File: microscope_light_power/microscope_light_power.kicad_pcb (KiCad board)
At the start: 2 copper layers, 50 x 40 mm, 37 parts, among them J1 MICROUSB, J2 5V175_out, J3 enable_switch, U1 MCP73871-2AA, U2 TPS61090

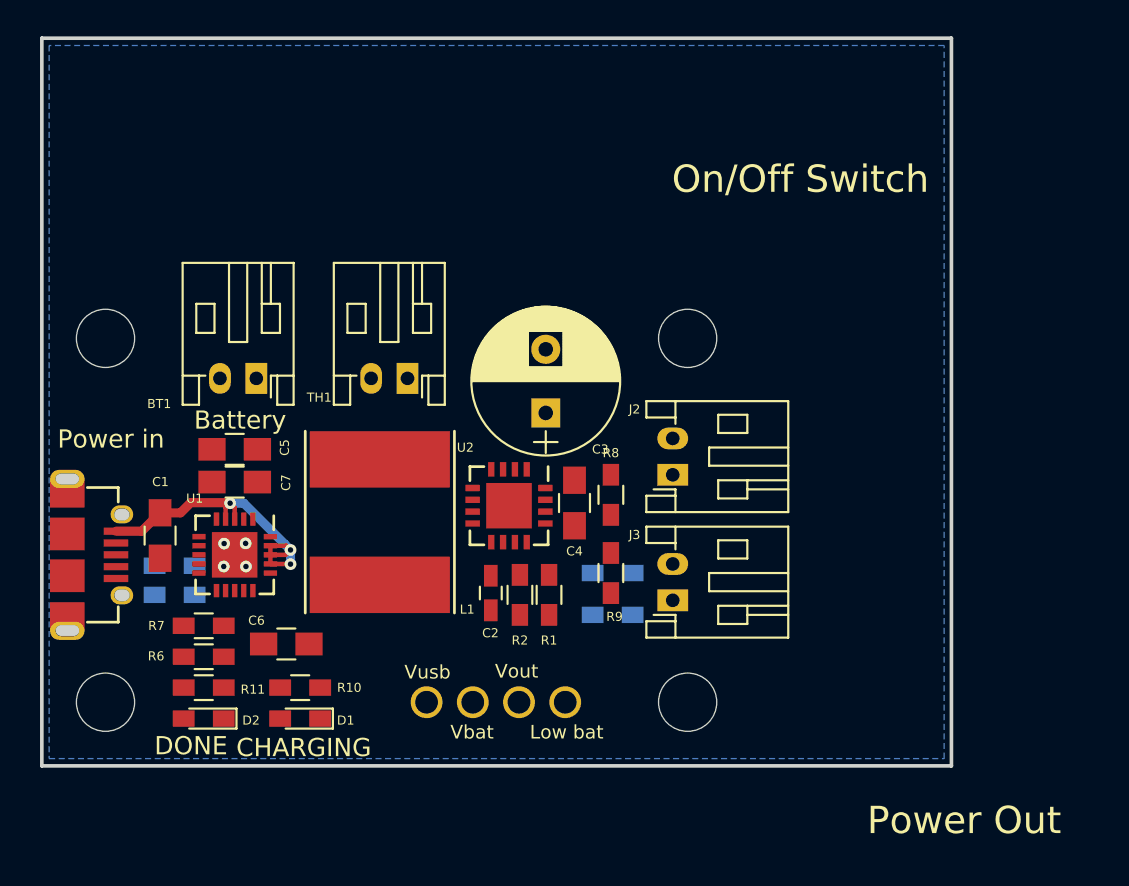
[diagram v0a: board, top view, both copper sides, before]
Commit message: Route the MCP73871
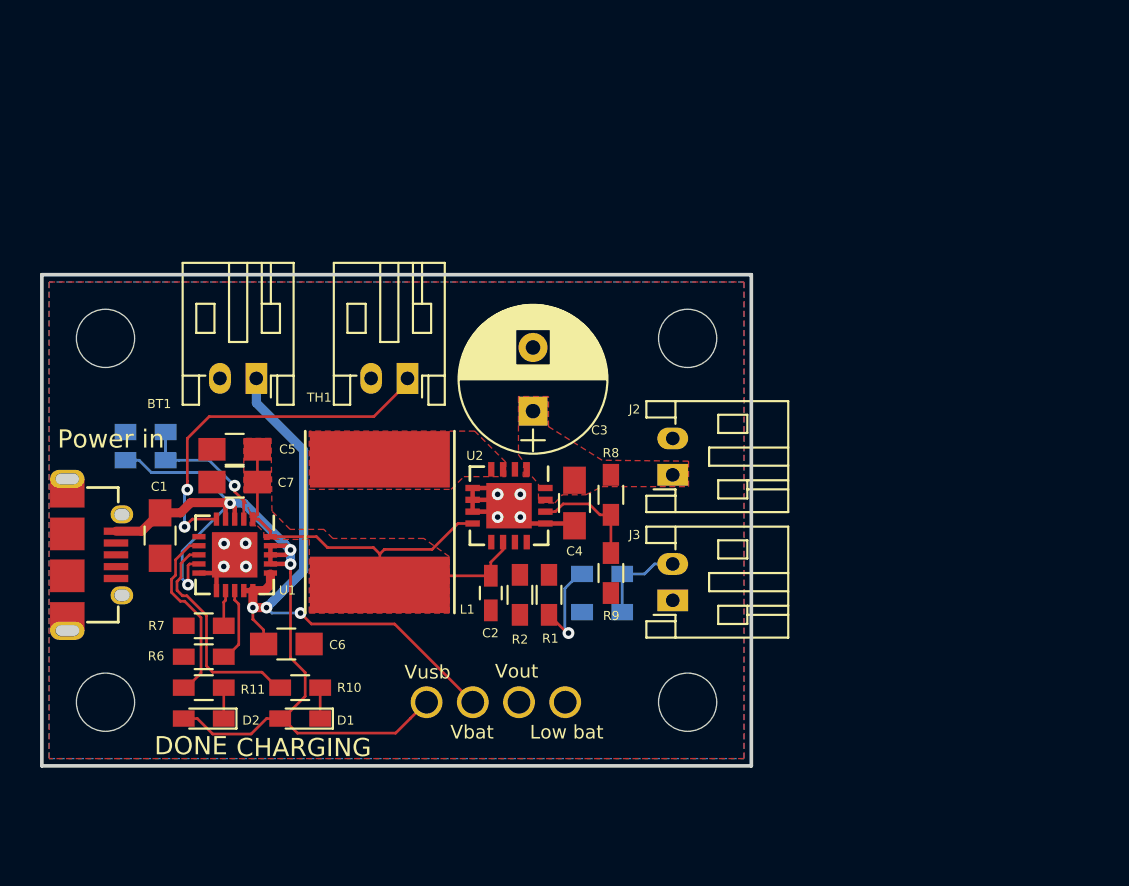
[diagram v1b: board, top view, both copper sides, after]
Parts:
- moved R5 9.09 mm to (105.7, 141.7)
- moved R4 6.02 mm to (105.7, 143.2)
- moved C3 0.71 mm to (127.0, 140.5)
- moved ROff3 0.60 mm to (130.8, 151.6), turned to 180 degrees
- moved ROn3 0.58 mm to (130.8, 149.4)
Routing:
- net /Vusb: track 18.7 -> 57.4 mm, vias 3 -> 4
- net /Vbat: track 0.00 -> 35.1 mm, vias 0 -> 3
- net /Vout: track 0.00 -> 33.1 mm, vias 0 -> 1
- net Net-(TH1-Pad1): track 0.00 -> 20.5 mm, vias 0 -> 2
- net GND: track 0.00 -> 13.2 mm, vias 4 -> 8
- net Net-(R10-Pad2): track 0.00 -> 12.3 mm
- net Net-(R11-Pad2): track 0.00 -> 10.0 mm
- net Net-(R4-Pad1): track 0.00 -> 7.97 mm, vias 0 -> 1
- net Net-(R8-Pad2): track 0.00 -> 6.12 mm
- net /enable: track 0.00 -> 5.11 mm
- net Net-(R6-Pad1): track 0.00 -> 4.16 mm
- net Net-(R7-Pad1): track 0.00 -> 1.98 mm
- net Net-(D2-Pad1): track 0.00 -> 1.70 mm
- net Net-(D1-Pad1): track 0.00 -> 1.70 mm
- added copper zone on F.Cu, net /5V175
- added copper zone on F.Cu, net /SW
- added copper zone on F.Cu, net /Vout
- added copper zone on F.Cu, net GND
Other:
- board size 50 x 40 mm -> 39 x 27 mm
- board text added: "10k NTC Thermistor"
- board text added: "5.175V@1.5A Out"
- board text added: "Jon Neal 2018 https://JonNeal.me https://github.com/microscope_light"
- board text removed: "Power Out"
